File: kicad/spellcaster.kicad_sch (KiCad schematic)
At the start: 38 parts, among them SW1 SW_Push, SW2 SW_Push, U1 nRF52820-QDxx, Y1 32k, Y2 Crystal_GND24

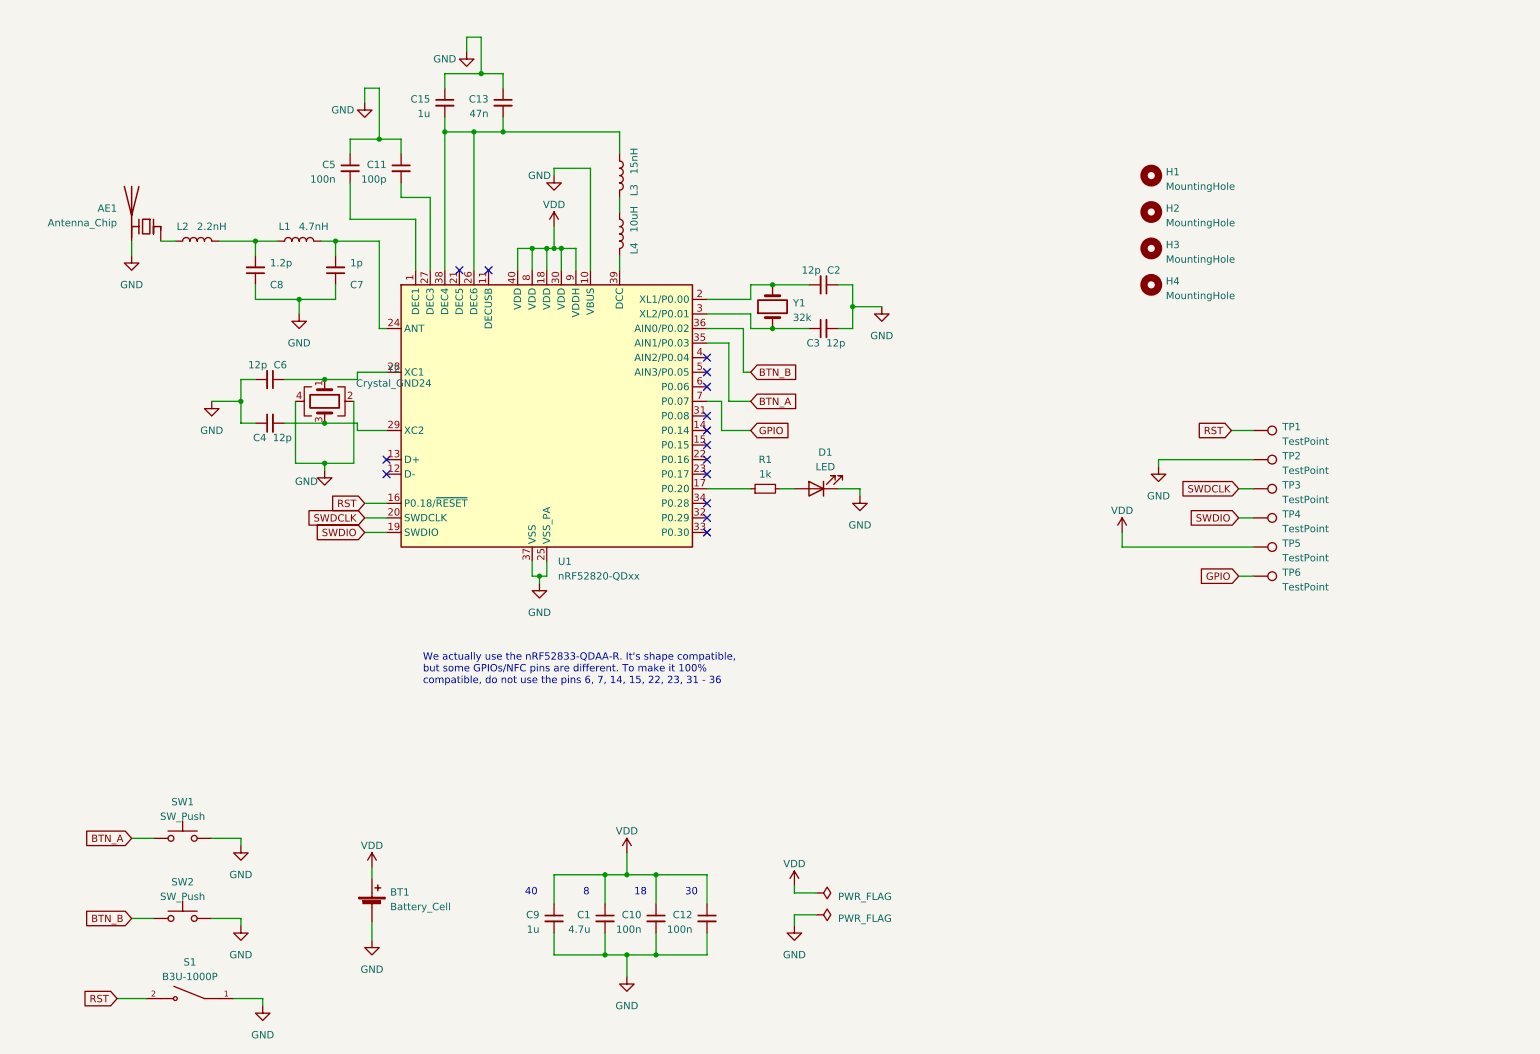
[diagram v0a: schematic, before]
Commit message: Initial routing
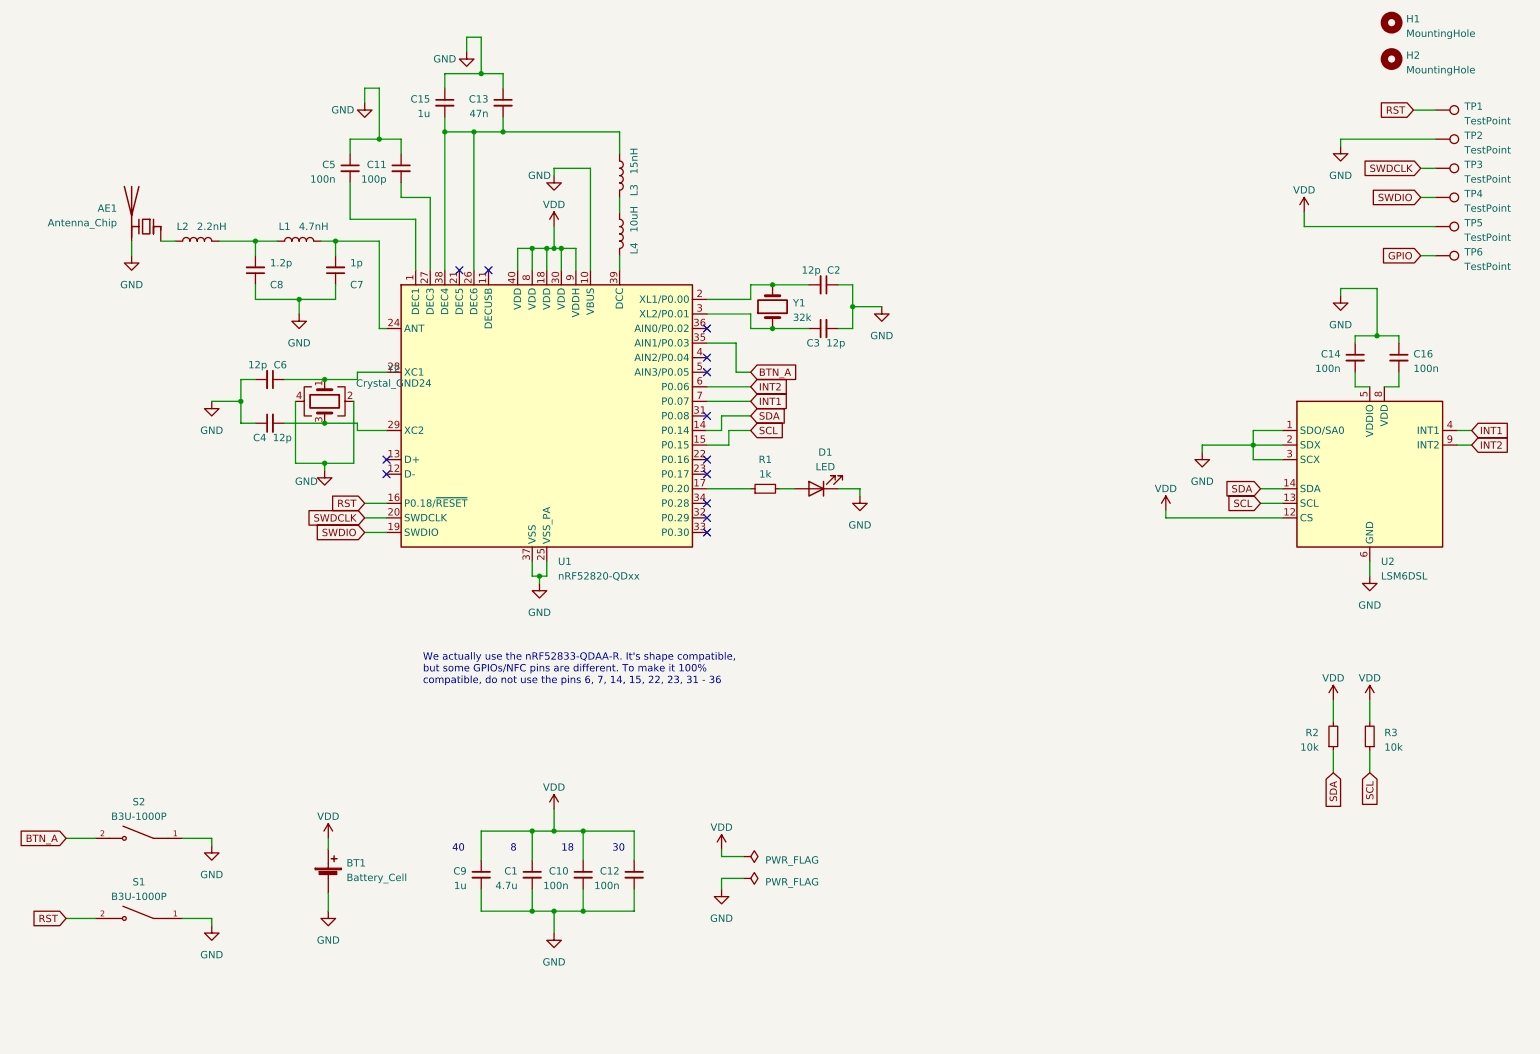
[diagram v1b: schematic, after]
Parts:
- removed H3, H4: MountingHole, MountingHole:MountingHole_2.2mm_M2_Pad_Via, symbol Mechanical:MountingHole
- removed SW1, SW2: SW_Push, Button_Switch_SMD:SW_SPST_PTS645, symbol Switch:SW_Push
- added C14, C16: 100n, Capacitor_SMD:C_0402_1005Metric, symbol Device:C_Small
- added R2, R3: 10k, Resistor_SMD:R_0402_1005Metric, symbol Device:R_Small
- added S2: B3U-1000P, Snapeda:SW_B3U-1000P, symbol Snapeda:B3U-1000P
- added U2: LSM6DSL, Package_LGA:LGA-14_3x2.5mm_P0.5mm_LayoutBorder3x4y, symbol Sensor_Motion:LSM6DSL
- BT1: footprint Battery:BatteryHolder_Keystone_3002_1x2032 -> Connector_Wire:SolderWire-0.5sqmm_1x02_P4.8mm_D0.9mm_OD2.3mm
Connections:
- net BTN_A: now also S2.2
- net GND: now also C14.1, C16.1, S2.1, U2.1 (SDO/SA0), U2.2 (SDX), U2.3 (SCX), U2.6 (GND), U2.7 (GND)
- net GPIO: no longer U1.7 (P0.07)
- net VDD: now also R2.2, R3.2, U2.12 (CS)
- net SDA: now reaches U1.14 (P0.14)
- net SDA: now also R2.1, U2.14 (SDA)
- net SCL: now reaches U1.15 (P0.15)
- net SCL: now also R3.1, U2.13 (SCL)
- net INT2: now reaches U1.6 (P0.06)
- net INT2: now also U2.9 (INT2)
- net BTN_B: no longer names the net of U1.36 (AIN0/P0.02)
- new net: C16.2, U2.8 (VDD)
- new net: C14.2, U2.5 (VDDIO)
- new net INT1: U1.7 (P0.07), U2.4 (INT1)
- no-connect marks 15 -> 13
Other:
- moved on the sheet: BT1, C1, C10, C12, C9, H1, H2, S1, TP1, TP2, TP3, TP4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
